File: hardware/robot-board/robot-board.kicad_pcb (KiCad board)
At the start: 4 copper layers, 69 x 99 mm, 136 parts, among them J1 Conn_01x09_Pin, J10 1x2_Screw, J11 1x2_Screw, J2 Barrel_Jack, J3 USB_C_Receptacle_USB2.0_14P, J4 Conn_01x03_Pin, J5 Conn_01x03_Pin, J6 Conn_01x03_Pin, J7 Conn_01x03_Pin, J8 1x2_Screw, J9 1x2_Screw, Q1 BSS138, Q2 BSS138, Q3 BSS138, Q4 BSS138, Q5 BSS138, Q6 BSS138, Q7 BSS138, Q8 BSS138, SW1 SW_SPST, SW2 SW_SPST, U1 ESP32-S3-WROOM-1, U2 LMR51450, U3 LMR51450, U4 TVS1400DRV, U5 TPS552892, U6 DRV8835, U7 DRV8835, U8 XL-SA3391SRWC, U9 STP08CP05M

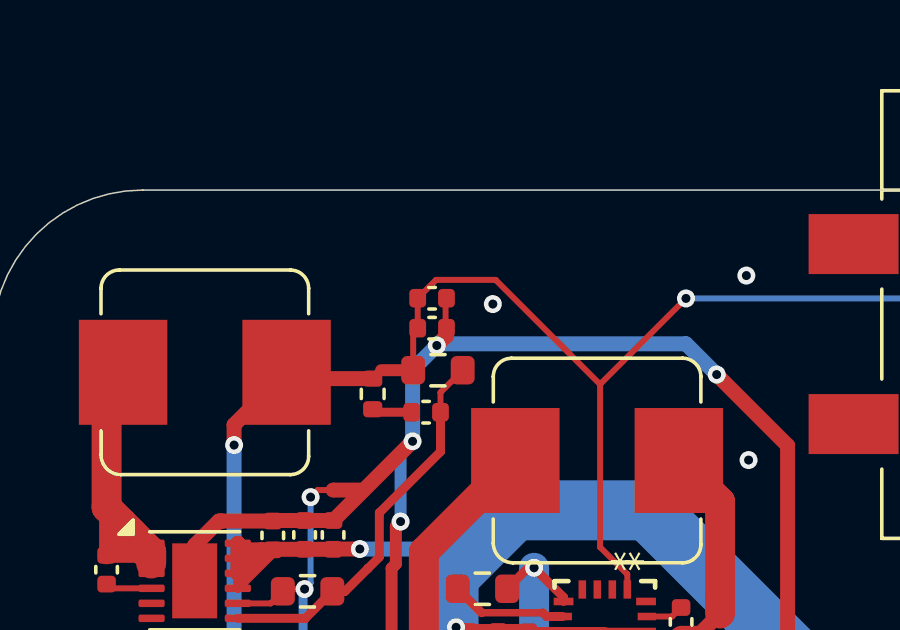
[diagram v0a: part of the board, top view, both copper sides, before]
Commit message: fixed the thingies
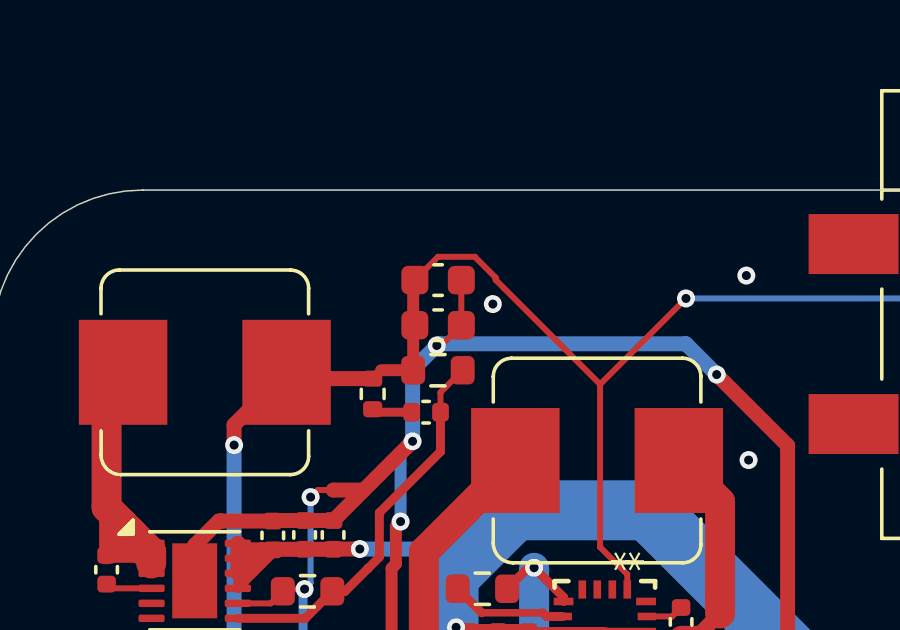
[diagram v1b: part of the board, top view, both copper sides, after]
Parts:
- C11, C13: footprint Capacitor_SMD:C_0402_1005Metric -> Capacitor_SMD:C_0603_1608Metric
- moved C11 0.64 mm to (50.9, 56.0)
- moved C13 0.22 mm to (50.9, 57.5)
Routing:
- net +3V3: track 240.3 -> 241.6 mm
- net PGND: track 69.1 -> 70.0 mm
